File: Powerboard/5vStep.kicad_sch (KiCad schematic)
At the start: 15 parts, among them U3 MP2338GTL-Z

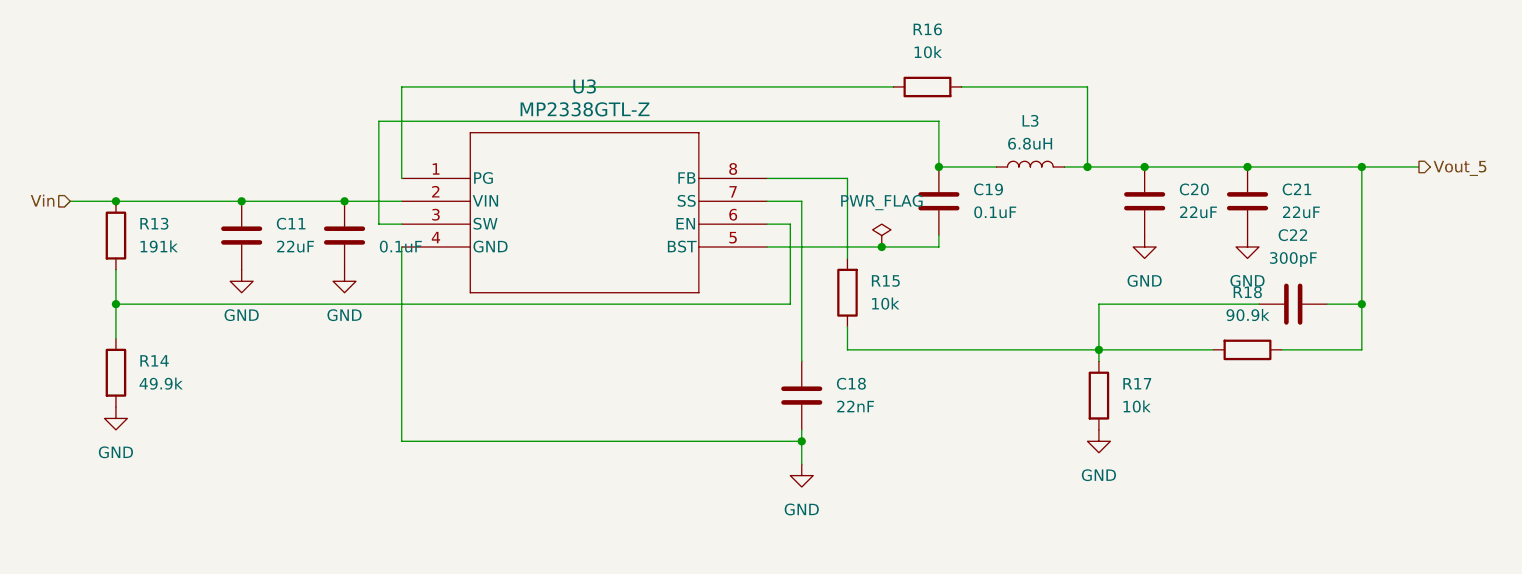
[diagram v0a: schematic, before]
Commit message: Updated
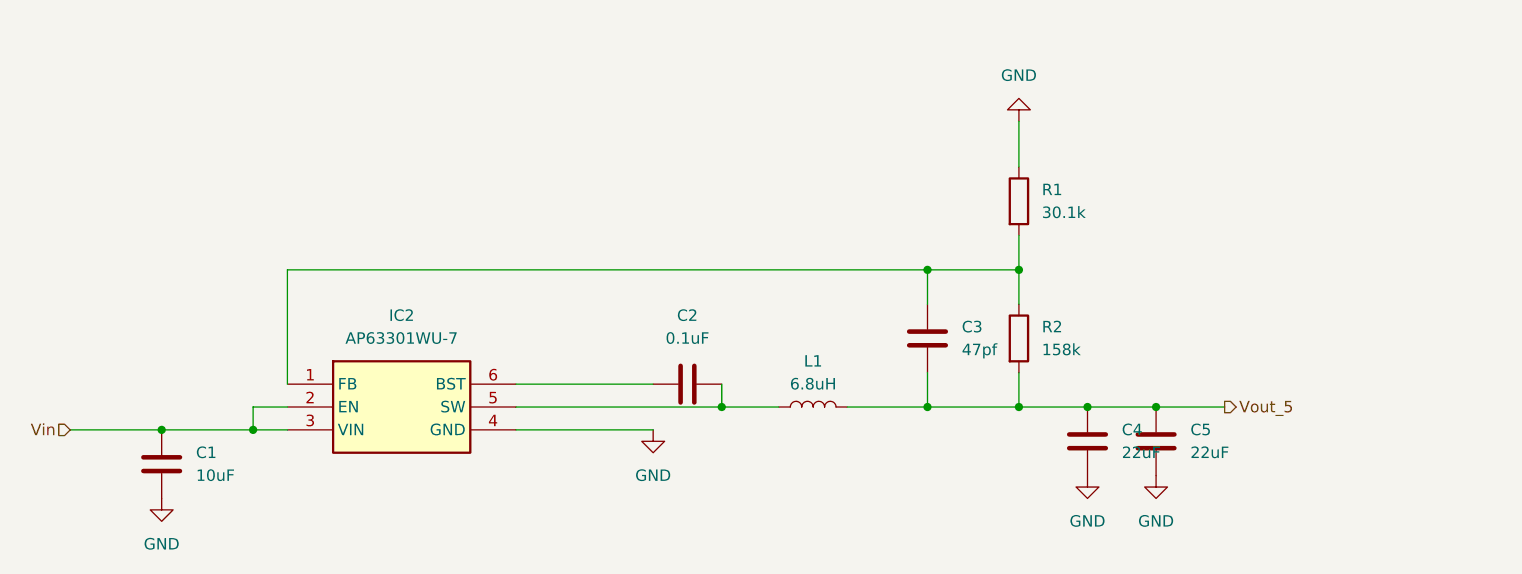
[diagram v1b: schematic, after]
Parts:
- removed C11, C20: 22uF, Capacitor_SMD:C_1206_3216Metric, symbol Device:C
- removed C17, C19: 0.1uF, Capacitor_SMD:C_0603_1608Metric, symbol Device:C
- removed C18: 22nF, Capacitor_SMD:C_0603_1608Metric, symbol Device:C
- removed C21: 22uF, Capacitor_SMD:C_0603_1608Metric, symbol Device:C
- removed C22: 300pF, Capacitor_SMD:C_0603_1608Metric, symbol Device:C
- removed L3: 6.8uH, Inductor_SMD:L_Bourns_SRP7028A_7.3x6.6mm, symbol Device:L
- removed R13: 191k, Resistor_SMD:R_0603_1608Metric, symbol Device:R
- removed R14: 49.9k, Resistor_SMD:R_0603_1608Metric, symbol Device:R
- removed R15, R16, R17: 10k, Resistor_SMD:R_0603_1608Metric, symbol Device:R
- removed R18: 90.9k, Resistor_SMD:R_0603_1608Metric, symbol Device:R
- removed U3: MP2338GTL-Z, MP2338GTL:SOT583_MP2338_MNP, symbol MP2338GTL:MP2338GTL-Z
- added C1: 10uF, Capacitor_SMD:C_1210_3225Metric, symbol Device:C
- added C2: 0.1uF, Capacitor_SMD:C_0603_1608Metric, symbol Device:C
- added C3: 47pf, Capacitor_SMD:C_0603_1608Metric, symbol Device:C
- added C4, C5: 22uF, Capacitor_SMD:C_1206_3216Metric, symbol Device:C
- added IC2: AP63301WU-7, AP63301WU:SOT95P280X100-6N, symbol AP63301WU:AP63301WU-7
- added L1: 6.8uH, Inductor_SMD:L_Bourns_SRP7028A_7.3x6.6mm, symbol Device:L
- added R1: 30.1k, Resistor_SMD:R_0603_1608Metric, symbol Device:R
- added R2: 158k, Resistor_SMD:R_0603_1608Metric, symbol Device:R
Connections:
- net GND: now also C1.2, C4.2, C5.2, IC2.4 (GND), R1.1
- net Vin: now also C1.1, IC2.2 (EN), IC2.3 (VIN)
- net Vout_5: now also C3.2, C4.1, C5.1, L1.2, R2.2
- new net: C2.2, IC2.5 (SW), L1.1
- new net: C3.1, IC2.1 (FB), R1.2, R2.1
- new net: C2.1, IC2.6 (BST)
